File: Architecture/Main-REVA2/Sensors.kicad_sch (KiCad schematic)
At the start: 19 parts, among them J12 Conn_01x04, J13 Conn_01x04, J15 Conn_01x04, J3 Conn_01x03, J4 Conn_01x04, J6 Conn_01x04, J7 Conn_01x06, J8 Conn_01x06, Q1 BS170

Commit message: Update_Sche
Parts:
- C16, C17, C18, C19, C2, C3, C6: footprint Capacitor_THT:C_Disc_D4.3mm_W1.9mm_P5.00mm -> CollecteurDonne:Capa disc radial 5.08mm
- R3, R6: footprint (none) -> CollecteurDonne:Résistance L10mm
- R5: footprint OptoDevice:R_LDR_10x8.5mm_P7.6mm_Vertical -> CollecteurDonne:Résistance L10mm
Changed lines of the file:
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@@
 			)
 		)
-		(property "Footprint" "OptoDevice:R_LDR_10x8.5mm_P7.6mm_Vertical"
+		(property "Footprint" "CollecteurDonne:Résistance L10mm"
 			(at 113.665 49.53 90)
 			(effects
@@
 			)
 		)
-		(property "Footprint" "Capacitor_THT:C_Disc_D4.3mm_W1.9mm_P5.00mm"
+		(property "Footprint" "CollecteurDonne:Capa disc radial 5.08mm"
 			(at 210.5152 100.33 0)
 			(effects
@@
 			)
 		)
-		(property "Footprint" "Capacitor_THT:C_Disc_D4.3mm_W1.9mm_P5.00mm"
+		(property "Footprint" "CollecteurDonne:Capa disc radial 5.08mm"
 			(at 136.8552 143.51 0)
 			(effects
@@
 			)
 		)
-		(property "Footprint" "Capacitor_THT:C_Disc_D4.3mm_W1.9mm_P5.00mm"
+		(property "Footprint" "CollecteurDonne:Capa disc radial 5.08mm"
 			(at 131.7752 101.6 0)
 			(effects
@@
 			)
 		)
-		(property "Footprint" "Capacitor_THT:C_Disc_D4.3mm_W1.9mm_P5.00mm"
+		(property "Footprint" "CollecteurDonne:Capa disc radial 5.08mm"
 			(at 65.7352 99.06 0)
 			(effects
@@
 			)
 		)
-		(property "Footprint" "Capacitor_THT:C_Disc_D4.3mm_W1.9mm_P5.00mm"
+		(property "Footprint" "CollecteurDonne:Capa disc radial 5.08mm"
 			(at 55.5752 143.51 0)
 			(effects
@@
 			)
 		)
-		(property "Footprint" ""
+		(property "Footprint" "CollecteurDonne:Résistance L10mm"
 			(at 169.164 63.754 90)
 			(effects
@@
 			)
 		)
-		(property "Footprint" ""
+		(property "Footprint" "CollecteurDonne:Résistance L10mm"
 			(at 110.236 59.944 90)
 			(effects
@@
 			)
 		)
-		(property "Footprint" "Capacitor_THT:C_Disc_D4.3mm_W1.9mm_P5.00mm"
+		(property "Footprint" "CollecteurDonne:Capa disc radial 5.08mm"
 			(at 218.1352 143.51 0)
 			(effects
@@
 			)
 		)
-		(property "Footprint" "Capacitor_THT:C_Disc_D4.3mm_W1.9mm_P5.00mm"
+		(property "Footprint" "CollecteurDonne:Capa disc radial 5.08mm"
 			(at 174.9552 55.88 0)
 			(effects

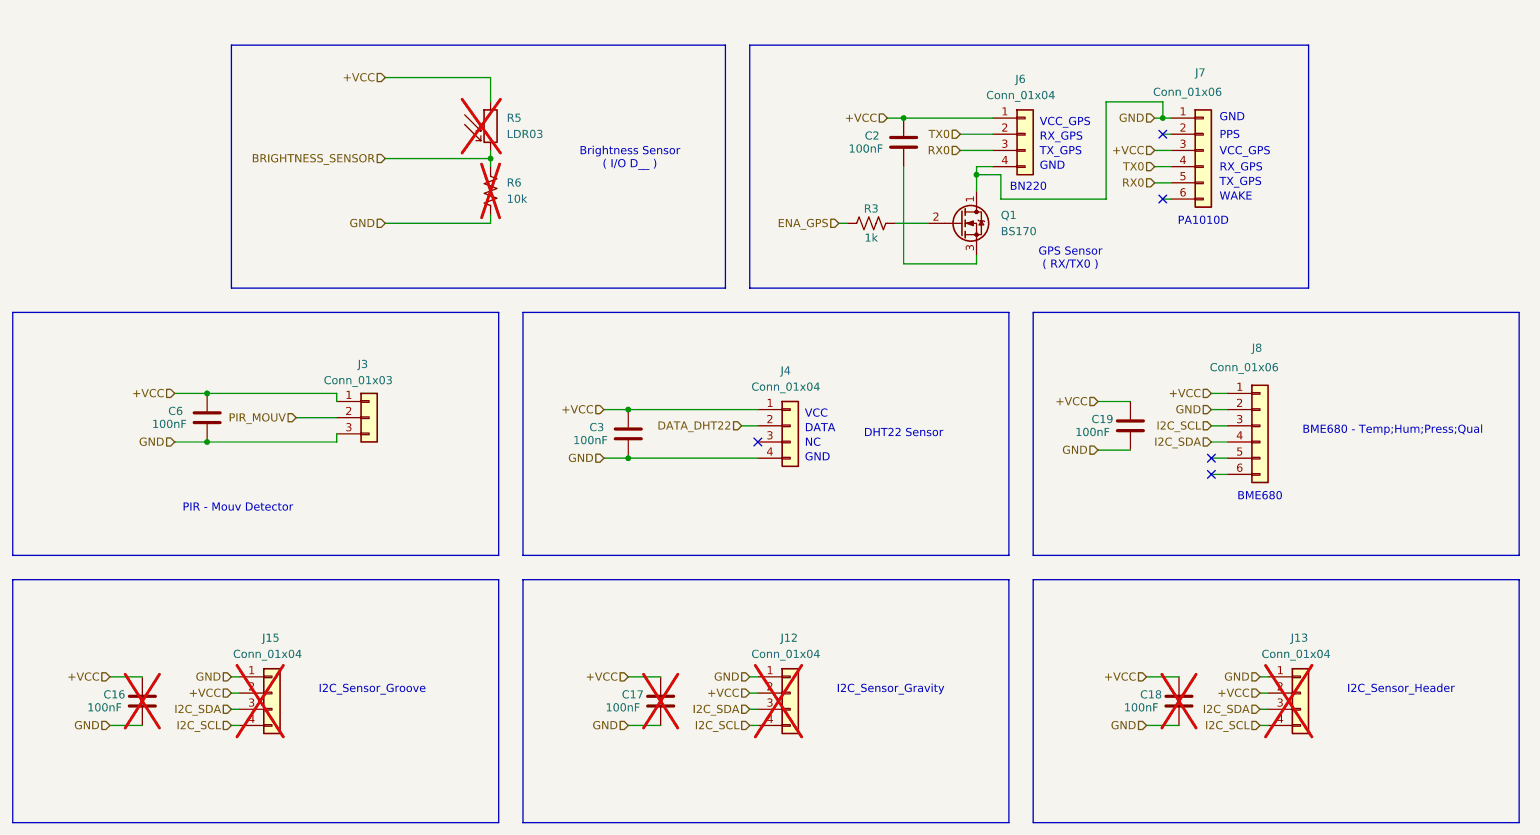
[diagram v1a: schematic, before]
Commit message: Update_Schematic_PCB
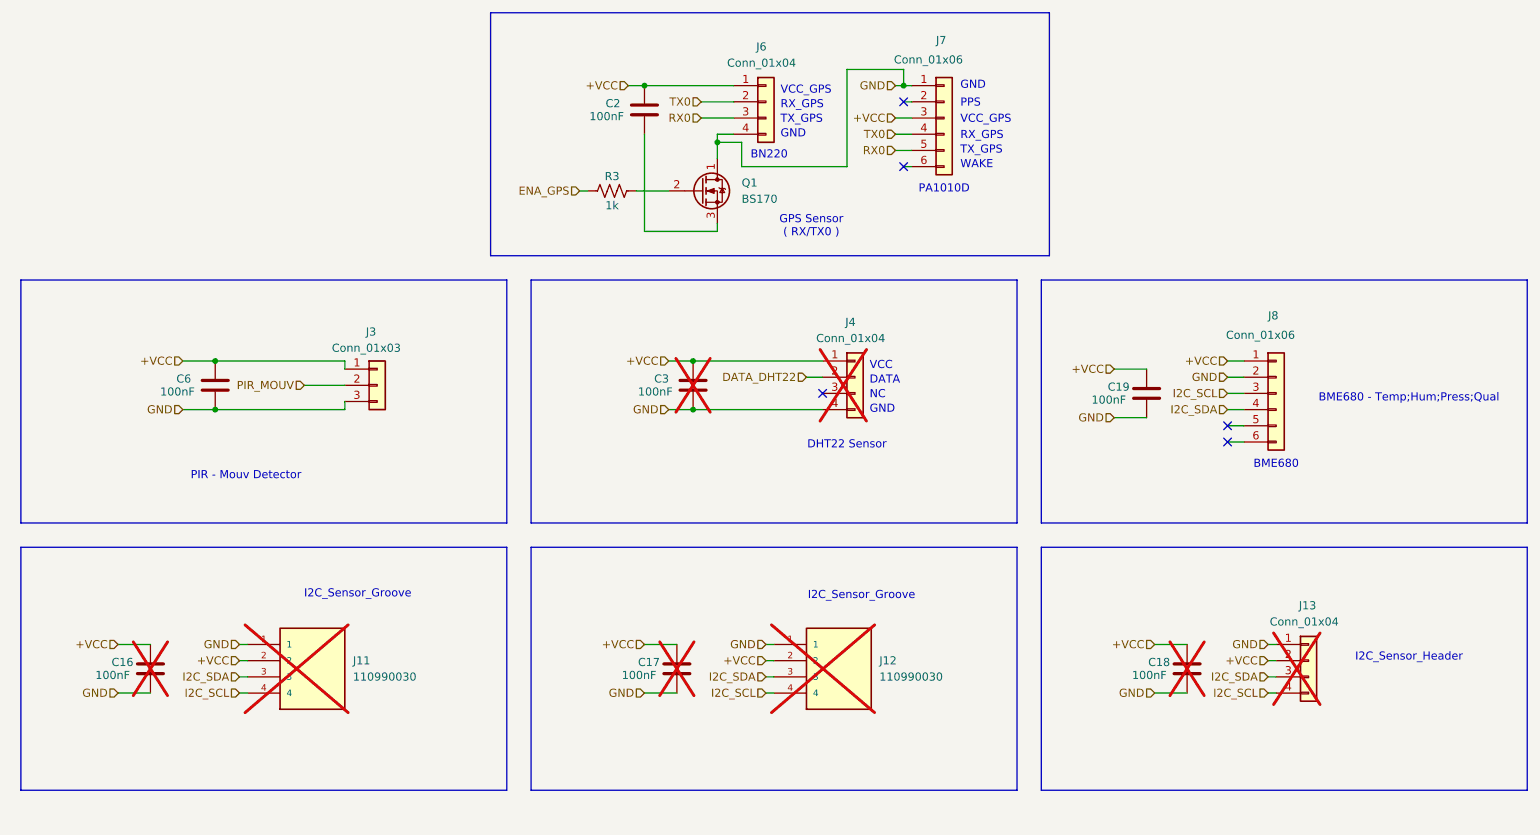
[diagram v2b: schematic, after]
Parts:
- removed J12, J15: Conn_01x04, symbol Connector_Generic:Conn_01x04
- removed R5: LDR03, CollecteurDonne:Résistance L10mm, symbol Sensor_Optical:LDR03
- removed R6: 10k, CollecteurDonne:Résistance L10mm, symbol Device:R_US
- added J11, J12: 110990030, 110990030:SEEED_110990030, symbol Grove:110990030
- C16, C17, C18, C19, C2, C6: footprint CollecteurDonne:Capa disc radial 5.08mm -> CollecteurDonne:C_Disc_D5.0mm_W2.5mm_P5.00mm
- C3: footprint CollecteurDonne:Capa disc radial 5.08mm -> CollecteurDonne:C_Disc_D5.0mm_W2.5mm_P5.00mm; now not fitted
- J13: footprint (none) -> Connector_PinHeader_2.54mm:PinHeader_1x04_P2.54mm_Vertical
- J4: now not fitted
- R3: footprint CollecteurDonne:Résistance L10mm -> CollecteurDonne:R_Axial_DIN0207_L6.3mm_D2.5mm_P10.16mm_Horizontal
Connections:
- net +VCC: now also J11.2, J12.2
- net GND: now also J11.1, J12.1
- net I2C_SCL: now also J11.4, J12.4
- net I2C_SDA: now also J11.3, J12.3
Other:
- note removed: "Brightness Sensor ( I/O D__ )"
- note removed: "I2C_Sensor_Gravity"
- moved on the sheet: C16, C17, C18, C19, C2, C6, J13, J3, J6, J7, J8, Q1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
